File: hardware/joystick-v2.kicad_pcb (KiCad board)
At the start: 2 copper layers, 45 x 25 mm, 23 parts, among them P1 CON-SENSOR2, P2 DEBUG, P3 BOOT, U1 XMC1XXX24, U3 JOYSTICK_BUTTON, U4 DRILL, U5 DRILL, U6 DRILL, U7 DRILL

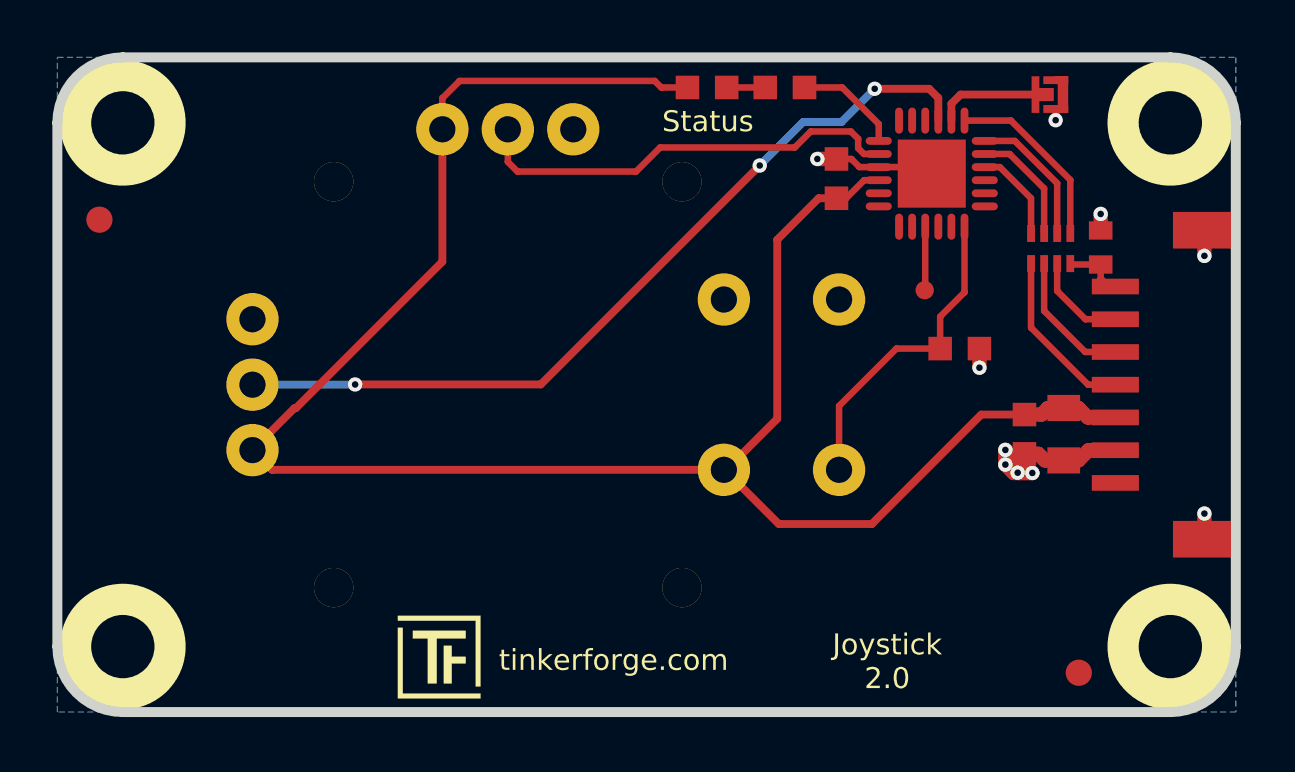
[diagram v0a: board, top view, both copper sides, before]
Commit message: Fix origin
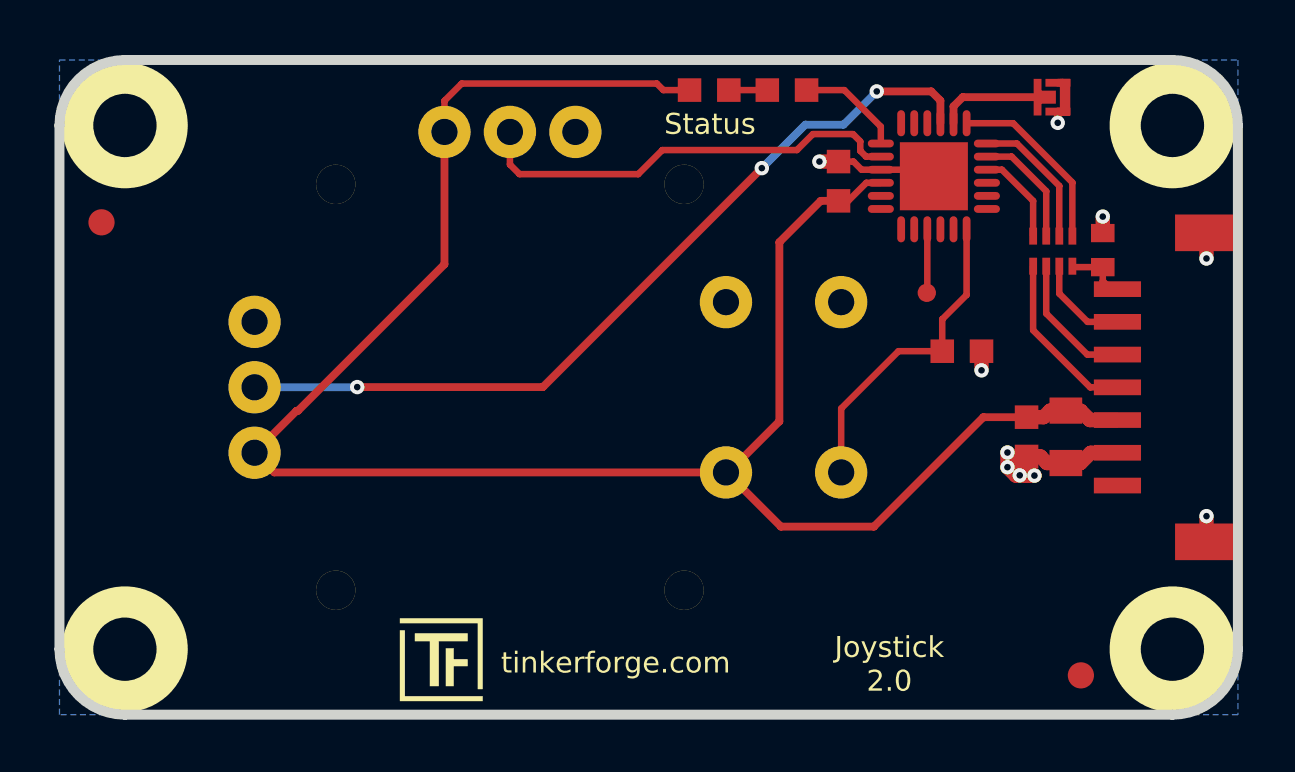
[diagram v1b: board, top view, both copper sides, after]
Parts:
- moved U1 0.13 mm to (155.1, 90.0)
- moved U3 0.13 mm to (138.9, 98.1)
- moved Fiducial_Mark 0.13 mm to (123.3, 91.8)
- moved Fiducial_Mark 0.13 mm to (160.7, 109.1)
- moved G*** 0.13 mm to (160.1, 98.1)
- moved VAL 0.13 mm to (146.5, 98.1)
- moved C2 0.13 mm to (151.4, 90.2)
- moved RP1 0.13 mm to (159.6, 92.9)
- moved Ref** 0.13 mm to (134.7, 106.9)
- moved U6 0.13 mm to (124.2, 108.1)
- moved U7 0.13 mm to (124.2, 88.1)
- moved C1 0.13 mm to (160.1, 100.0)
- moved C3 0.13 mm to (161.5, 92.9)
- moved C4 0.13 mm to (158.6, 100.0)
- moved D1 0.13 mm to (146.5, 86.8)
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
